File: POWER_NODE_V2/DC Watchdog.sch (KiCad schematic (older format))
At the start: 2 parts, among them J8 CONN_01X01

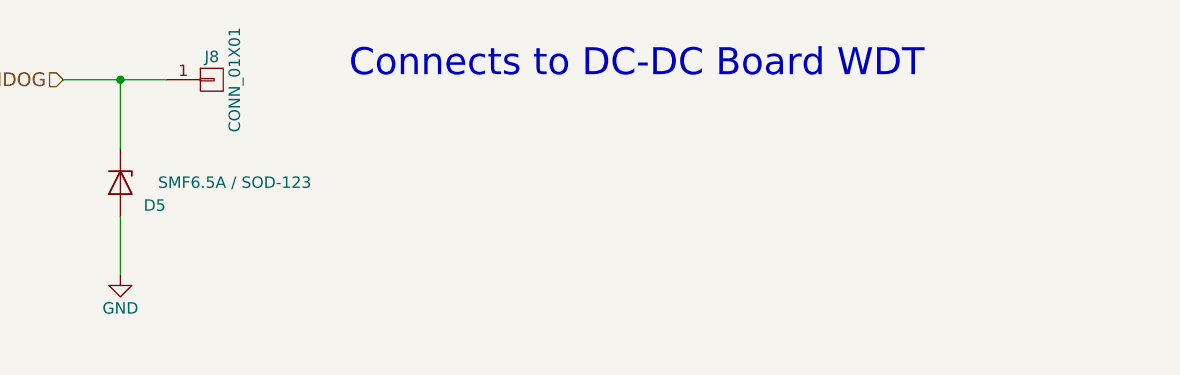
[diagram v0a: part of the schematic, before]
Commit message: All modelled, schematics and mechanical just need a double check
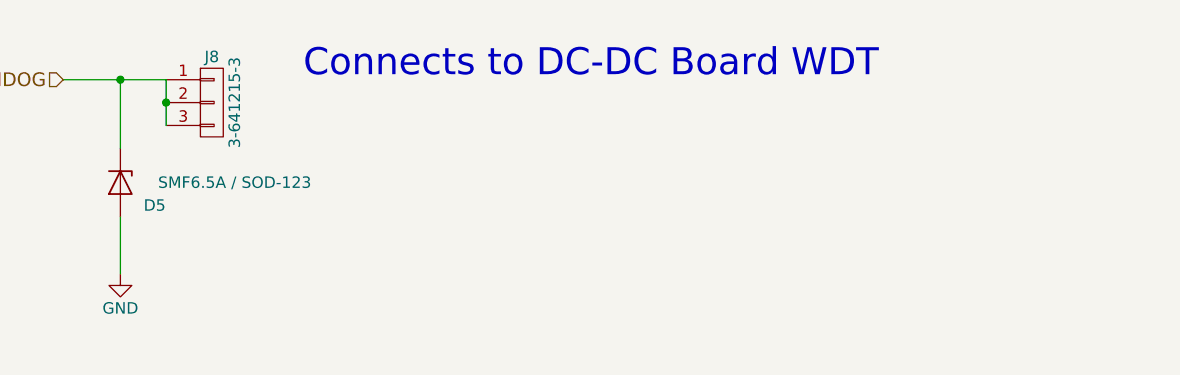
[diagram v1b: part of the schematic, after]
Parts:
- removed J8: CONN_01X01, Pin_Headers:Pin_Header_Straight_1x01_Pitch2.54mm, symbol CONN_01X01
- added J8: 3-641215-3, rLoop_Footprints:3-641215-3_3Pin_Latching_Header, symbol CONN_01X03
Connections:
- net DC_WATCHDOG: now also J8.1 (P1), J8.2 (P2), J8.3 (P3)
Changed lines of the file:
@@
 Text HLabel 4050 3450 0    60   Input ~ 0
 DC_WATCHDOG
-$Comp
-L CONN_01X01 J8
-U 1 1 5951AEA4
-P 4700 3450
-F 0 "J8" H 4700 3550 50  0000 C CNN
-F 1 "CONN_01X01" V 4800 3450 50  0000 C CNN
-F 2 "Pin_Headers:Pin_Header_Straight_1x01_Pitch2.54mm" H 4700 3450 50  0001 C CNN
-F 3 "" H 4700 3450 50  0001 C CNN
-	1    4700 3450
-	1    0    0    -1
-$EndComp
 Wire Wire Line
 	4050 3450 4500 3450
@@
 Connection ~ 4300 3450
 $Comp
-L GND #PWR096
+L GND #PWR095
 U 1 1 5952668C
 P 4300 4300
-F 0 "#PWR096" H 4300 4050 50  0001 C CNN
+F 0 "#PWR095" H 4300 4050 50  0001 C CNN
 F 1 "GND" H 4300 4150 50  0000 C CNN
 F 2 "" H 4300 4300 50  0001 C CNN
@@
 Wire Wire Line
 	4300 4300 4300 4050
-Text Notes 5300 3450 0    118  ~ 0
+Text Notes 5100 3450 0    118  ~ 0
 Connects to DC-DC Board WDT
 Text Notes 6550 7200 0    197  ~ 0
 DC Watchdog
+$Comp
+L CONN_01X03 J8
+U 1 1 595ADFEE
+P 4700 3550
+F 0 "J8" H 4700 3750 50  0000 C CNN
+F 1 "3-641215-3" V 4800 3550 50  0000 C CNN
+F 2 "rLoop_Footprints:3-641215-3_3Pin_Latching_Header" H 4700 3550 50  0001 C CNN
+F 3 "" H 4700 3550 50  0001 C CNN
+	1    4700 3550
+	1    0    0    -1
+$EndComp
+Wire Wire Line
+	4500 3450 4500 3650
+Connection ~ 4500 3550
 $EndSCHEMATC
